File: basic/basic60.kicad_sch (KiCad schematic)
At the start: 137 parts, among them J1 Conn_ARM_SW, J2 AudioJack3_Ground, J3 AudioJack3_Ground, J4 BAT, SW1 SW_Push, SW10 SW_Push, SW11 SW_Push, SW12 SW_Push, SW13 SW_Push, SW14 SW_Push, SW15 SW_Push, SW16 SW_Push, SW17 SW_Push, SW18 SW_Push, SW19 SW_Push, SW2 SW_Push, SW20 SW_Push, SW21 SW_Push, SW22 SW_Push, SW23 SW_Push, SW24 SW_Push, SW25 SW_Push, SW26 SW_Push, SW27 SW_Push, SW28 SW_Push, SW29 SW_Push, SW3 SW_Push, SW30 SW_Push, SW31 SW_Push, SW32 SW_Push, SW33 SW_Push, SW34 SW_Push, SW35 SW_Push, SW36 SW_Push, SW37 SW_Push, SW38 SW_Push, SW39 SW_Push, SW4 SW_Push, SW40 SW_Push, SW41 SW_Push, SW42 SW_Push, SW43 SW_Push, SW44 SW_Push, SW45 SW_Push, SW46 SW_Push, SW47 SW_Push, SW48 SW_Push, SW49 SW_Push, SW5 SW_Push, SW50 SW_Push, SW51 SW_Push, SW52 SW_Push, SW53 SW_Push, SW54 SW_Push, SW55 SW_Push, SW56 SW_Push, SW57 SW_Push, SW58 SW_Push, SW59 SW_Push, SW6 SW_Push, SW60 SW_Push, SW7 SW_Push, SW8 SW_Push, SW9 SW_Push, U1 Seeeduino Xiao nRF52840, U2 PCA9555PW

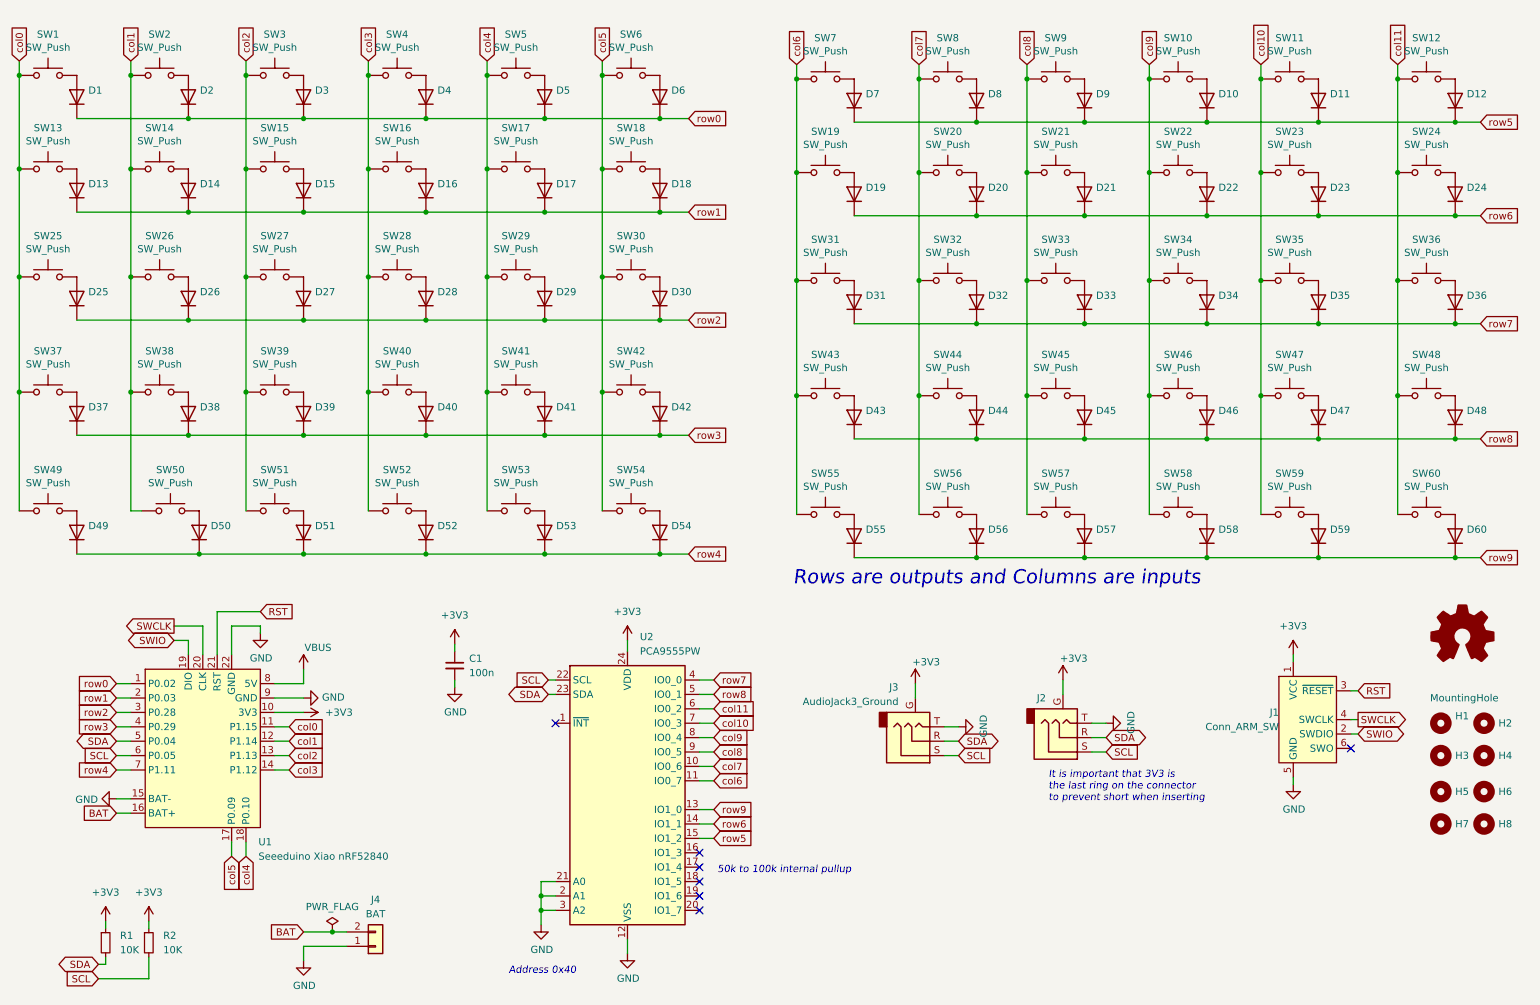
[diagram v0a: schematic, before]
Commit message: finish pcb
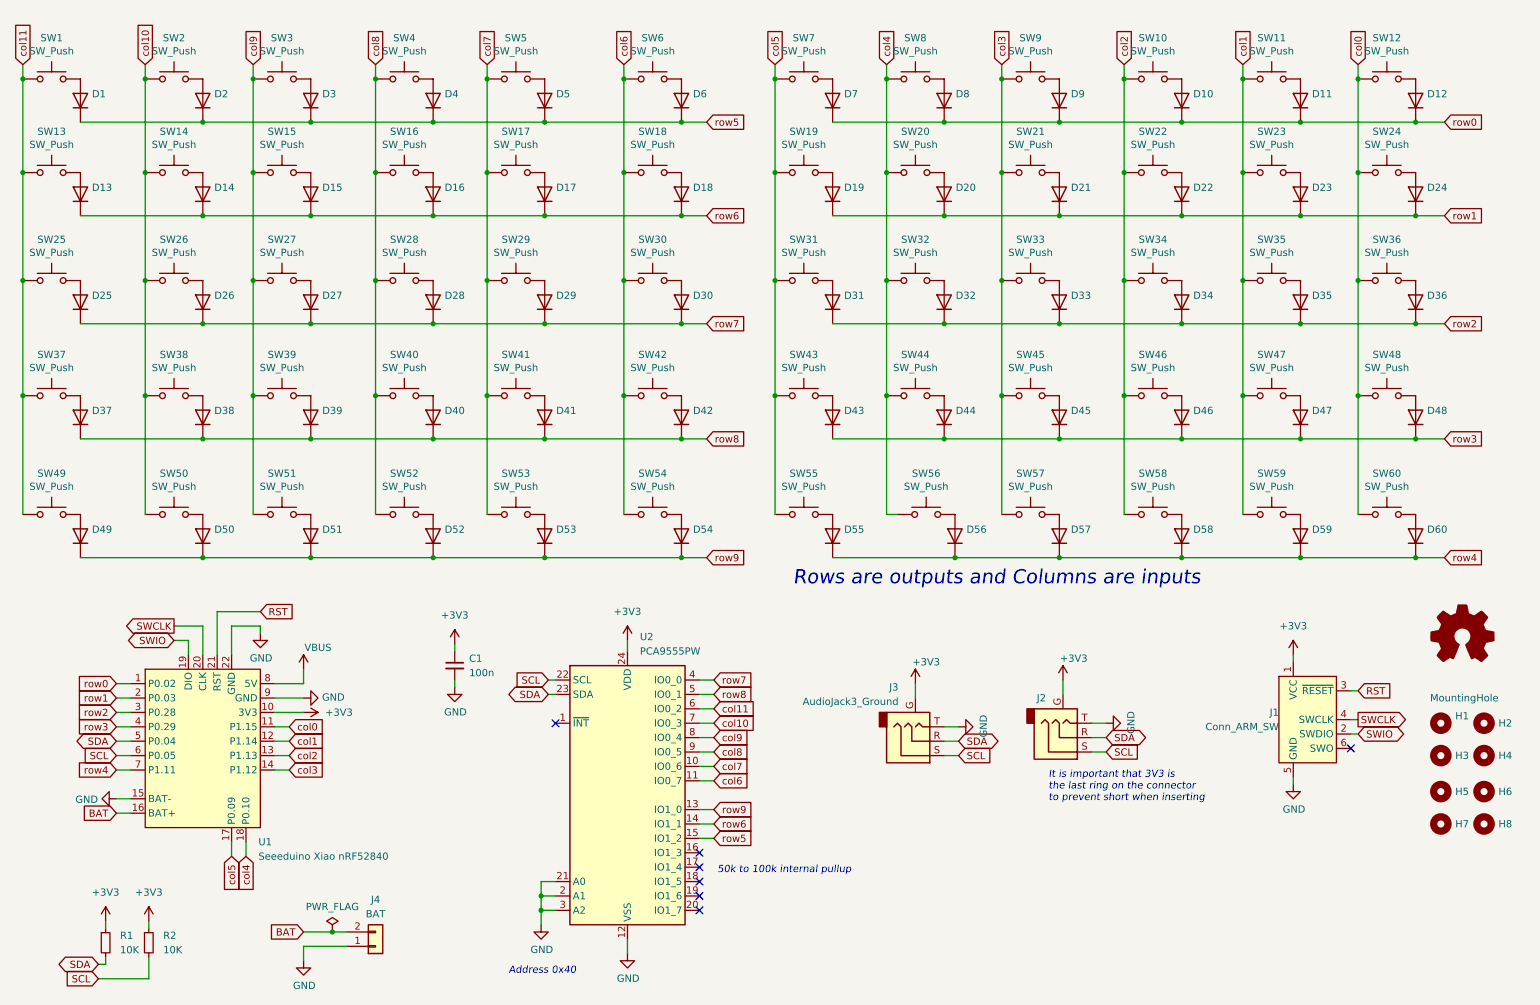
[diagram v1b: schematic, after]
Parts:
- renumbered D7 to D1, D4 to D10, D5 to D11, D6 to D12, D19 to D13, D20 to D14, D21 to D15, D22 to D16, D23 to D17, D24 to D18, D13 to D19, D8 to D2, D14 to D20, D15 to D21, D16 to D22, D17 to D23, D18 to D24, D31 to D25, D32 to D26, D33 to D27, D34 to D28, D35 to D29, D9 to D3, D36 to D30, D25 to D31, D26 to D32, D27 to D33, D28 to D34, D29 to D35, D30 to D36, D43 to D37, D44 to D38, D45 to D39, D10 to D4, D46 to D40, D47 to D41, D48 to D42, D37 to D43, D38 to D44, D39 to D45, D40 to D46, D41 to D47, D42 to D48, D55 to D49, D11 to D5, D56 to D50, D57 to D51, D58 to D52, D59 to D53, D60 to D54, D49 to D55, D50 to D56, D51 to D57, D52 to D58, D53 to D59, D12 to D6, D54 to D60, D1 to D7, D2 to D8, D3 to D9, SW7 to SW1, SW4 to SW10, SW5 to SW11, SW6 to SW12, SW19 to SW13, SW20 to SW14, SW21 to SW15, SW22 to SW16, SW23 to SW17, SW24 to SW18, SW13 to SW19, SW8 to SW2, SW14 to SW20, SW15 to SW21, SW16 to SW22, SW17 to SW23, SW18 to SW24, SW31 to SW25, SW32 to SW26, SW33 to SW27, SW34 to SW28, SW35 to SW29, SW9 to SW3, SW36 to SW30, SW25 to SW31, SW26 to SW32, SW27 to SW33, SW28 to SW34, SW29 to SW35, SW30 to SW36, SW43 to SW37, SW44 to SW38, SW45 to SW39, SW10 to SW4, SW46 to SW40, SW47 to SW41, SW48 to SW42, SW37 to SW43, SW38 to SW44, SW39 to SW45, SW40 to SW46, SW41 to SW47, SW42 to SW48, SW55 to SW49, SW11 to SW5, SW56 to SW50, SW57 to SW51, SW58 to SW52, SW59 to SW53, SW60 to SW54, SW49 to SW55, SW50 to SW56, SW51 to SW57, SW52 to SW58, SW53 to SW59, SW12 to SW6, SW54 to SW60, SW1 to SW7, SW2 to SW8, SW3 to SW9
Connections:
- net col0: now also SW12.1, SW24.1, SW36.1, SW48.1, SW60.1; no longer SW19.1, SW31.1, SW43.1, SW55.1, SW7.1
- net col1: now also SW11.1, SW23.1, SW35.1, SW47.1, SW59.1; no longer SW20.1, SW32.1, SW44.1, SW56.1, SW8.1
- net col10: now also SW14.1, SW2.1, SW26.1, SW38.1, SW50.1; no longer SW17.1, SW29.1, SW41.1, SW5.1, SW53.1
- net col11: now also SW1.1, SW13.1, SW25.1, SW37.1, SW49.1; no longer SW18.1, SW30.1, SW42.1, SW54.1, SW6.1
- net col2: now also SW10.1, SW22.1, SW34.1, SW46.1, SW58.1; no longer SW21.1, SW33.1, SW45.1, SW57.1, SW9.1
- net col3: now also SW21.1, SW33.1, SW45.1, SW57.1, SW9.1; no longer SW10.1, SW22.1, SW34.1, SW46.1, SW58.1
- net col4: now also SW20.1, SW32.1, SW44.1, SW56.1, SW8.1; no longer SW11.1, SW23.1, SW35.1, SW47.1, SW59.1
- net col5: now also SW19.1, SW31.1, SW43.1, SW55.1, SW7.1; no longer SW12.1, SW24.1, SW36.1, SW48.1, SW60.1
- net col6: now also SW18.1, SW30.1, SW42.1, SW54.1, SW6.1; no longer SW1.1, SW13.1, SW25.1, SW37.1, SW49.1
- net col7: now also SW17.1, SW29.1, SW41.1, SW5.1, SW53.1; no longer SW14.1, SW2.1, SW26.1, SW38.1, SW50.1
- net col8: now also SW16.1, SW28.1, SW4.1, SW40.1, SW52.1; no longer SW15.1, SW27.1, SW3.1, SW39.1, SW51.1
- net col9: now also SW15.1, SW27.1, SW3.1, SW39.1, SW51.1; no longer SW16.1, SW28.1, SW4.1, SW40.1, SW52.1
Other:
- moved on the sheet: D1, D10, D11, D12, D13, D14, D15, D16, D17, D18, D19, D2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
